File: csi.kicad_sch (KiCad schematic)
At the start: 69 parts, among them J10 Conn_01x22_MountingPin, J11 Conn_01x22_MountingPin, J8 Conn_01x22_MountingPin, J9 Conn_01x22_MountingPin, U16 PI4MSD5V9548AZDEX, U17 AP22615A, U18 AP22615A, U19 AP22615A, U20 AP22615A, U21 NTS0102, U22 NTS0102

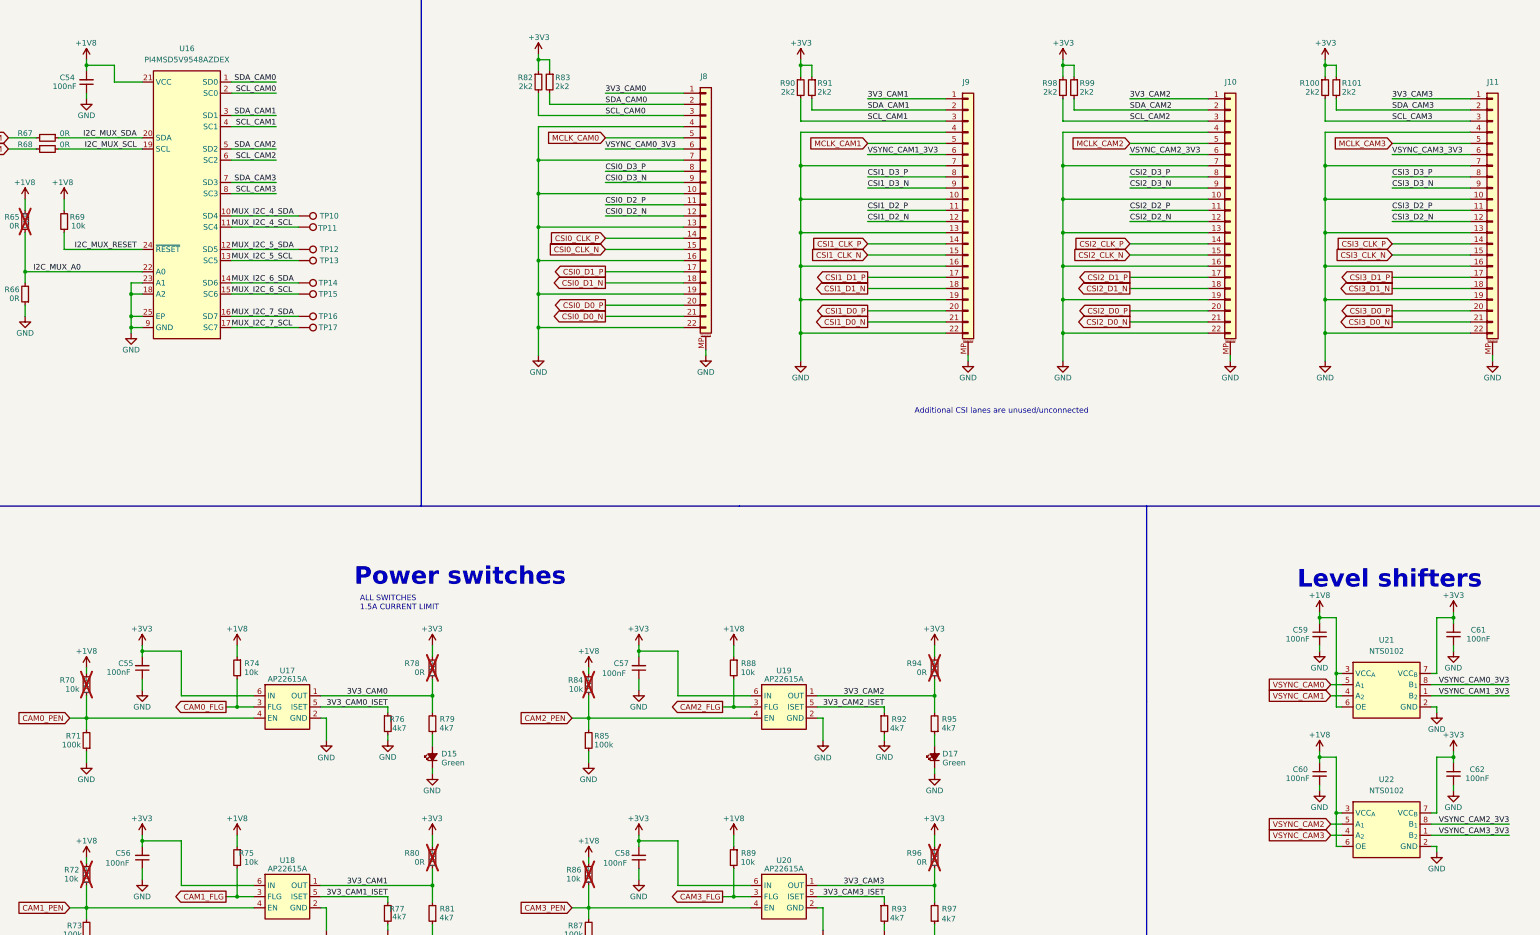
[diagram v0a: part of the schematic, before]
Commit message: Final BOM changes, gerbers
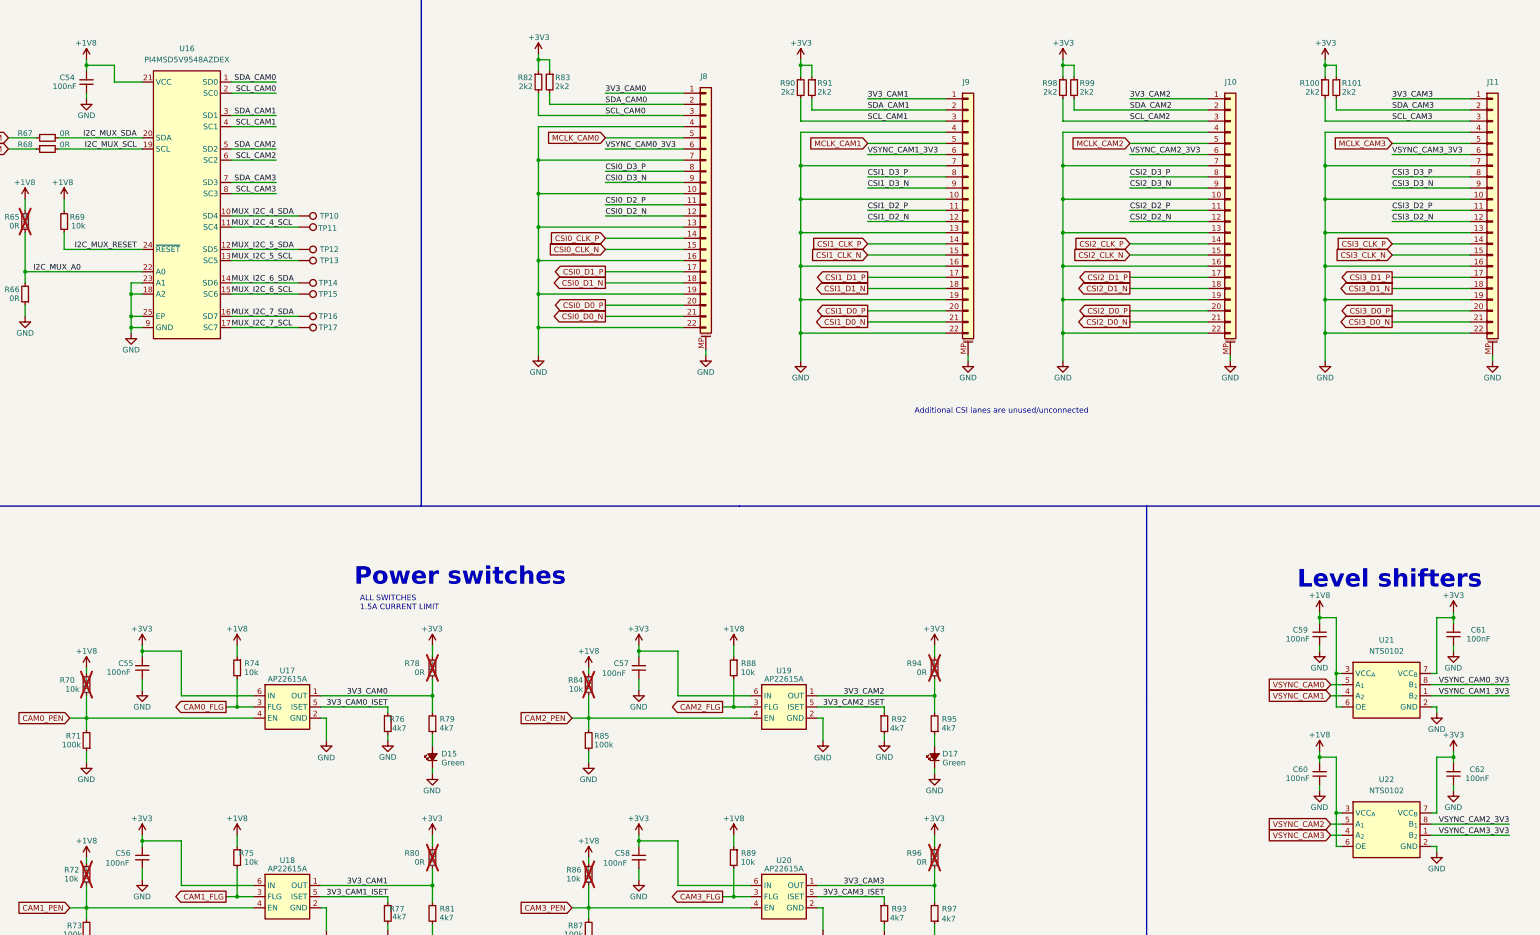
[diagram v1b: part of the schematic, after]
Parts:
- C54, C55, C56, C57, C58, C59, C60, C61, C62: LCSC (none) -> C14663
- D15, D16, D17, D18: LCSC (none) -> C12065
- R100, R101, R82, R83, R90, R91, R98, R99: LCSC (none) -> C4190
- R65, R66, R67, R68: LCSC (none) -> C17168
- R69, R70, R72, R74, R75, R84, R86, R88, R89: LCSC (none) -> C25804
- R71, R73, R85, R87: LCSC (none) -> C25803
- R76, R77, R79, R81, R92, R93, R95, R97: LCSC (none) -> C23162
- R78, R80, R94, R96: LCSC (none) -> C21189
- U16: LCSC (none) -> C2674581
- U17, U18, U19, U20: LCSC (none) -> C2680357
- U21, U22: LCSC (none) -> C2687851
